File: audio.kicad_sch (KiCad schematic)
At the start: 18 parts, among them J1 USB4105-GF-A, U1 PCM5102APW, U2 TPA6130A2RTJR, U3 DEV-15583

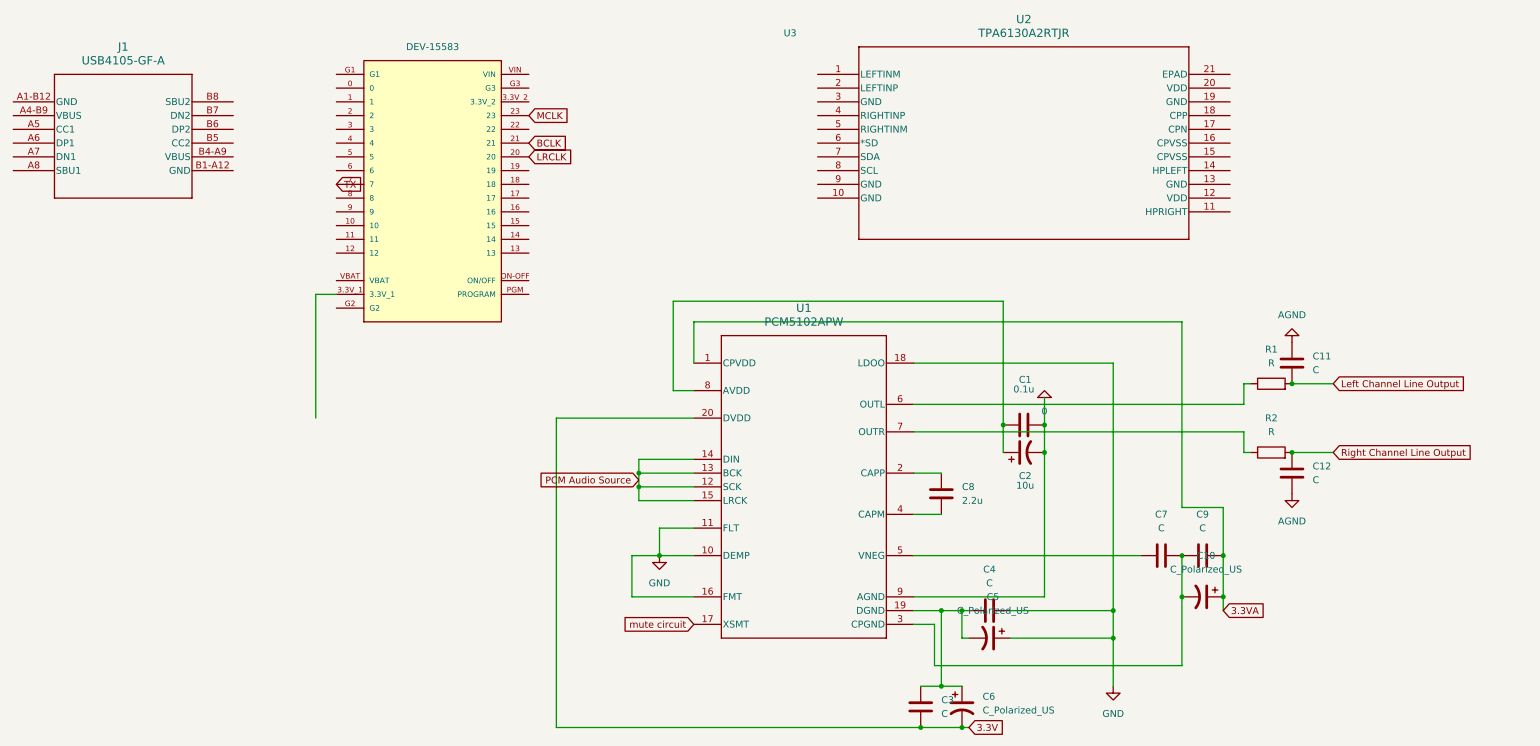
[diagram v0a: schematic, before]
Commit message: Amplifier reference values
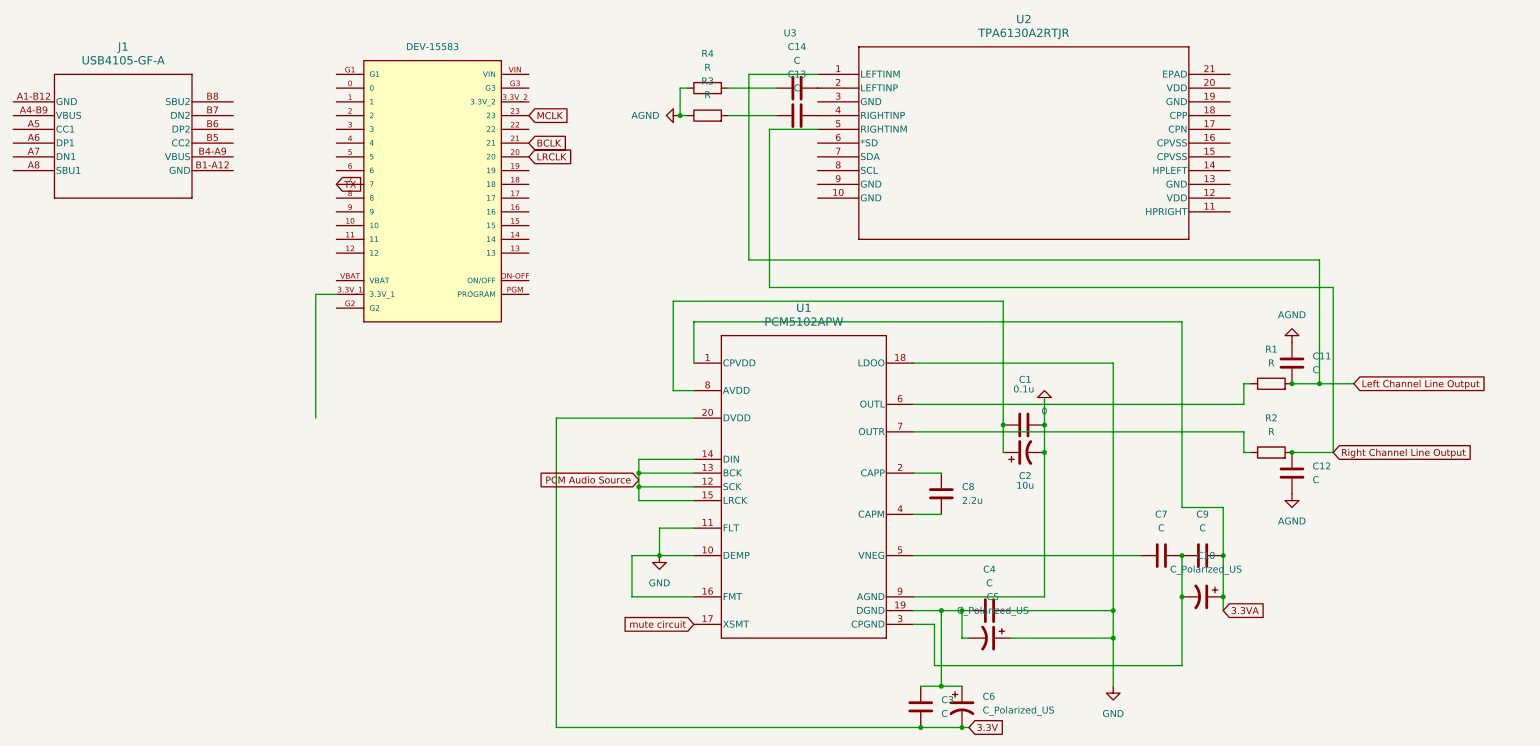
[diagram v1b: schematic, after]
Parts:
- added C13, C14: C, symbol Device:C
- added R3, R4: R, symbol Device:R
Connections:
- net AGND: now also R3.1, R4.1
- net Left Channel Line Output: now also U2.1 (LEFTINM)
- net Right Channel Line Output: now also U2.5 (RIGHTINM)
- net at U2.2 (LEFTINP): now also C14.2
- net at U2.4 (RIGHTINP): now also C13.2
- new net: C14.1, R4.2
- new net: C13.1, R3.2

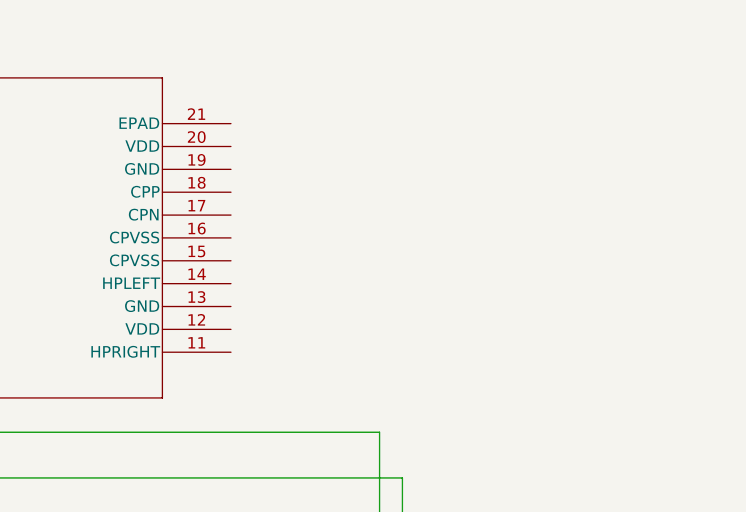
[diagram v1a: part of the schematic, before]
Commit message: Amplifier stuff
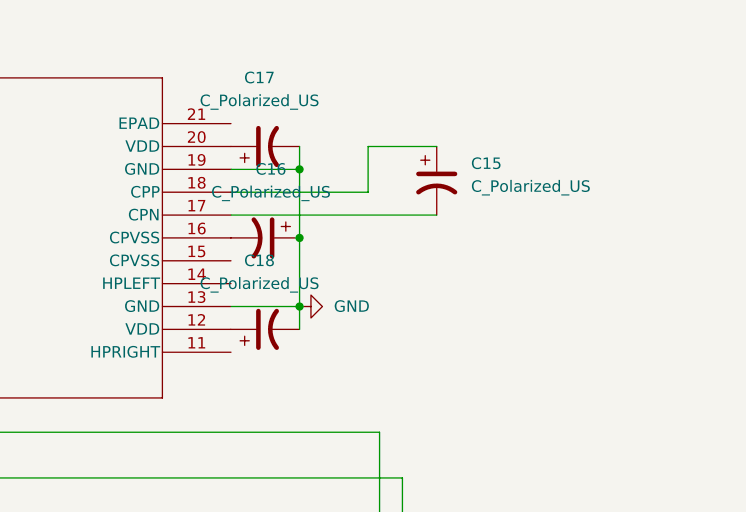
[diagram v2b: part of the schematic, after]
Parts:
- added C15, C16, C17, C18: C_Polarized_US, symbol Device:C_Polarized_US
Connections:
- net GND: now also U2.13 (GND), U2.19 (GND), C16.1, C17.2, C18.2
- net at U2.12 (VDD): now also C18.1
- net at U2.16 (CPVSS): now also C16.2
- net at U2.17 (CPN): now also C15.2
- net at U2.18 (CPP): now also C15.1
- net at U2.20 (VDD): now also C17.1
